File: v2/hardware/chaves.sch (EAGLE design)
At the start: 75 parts, among them IC1 40106N, IC2 7805DT

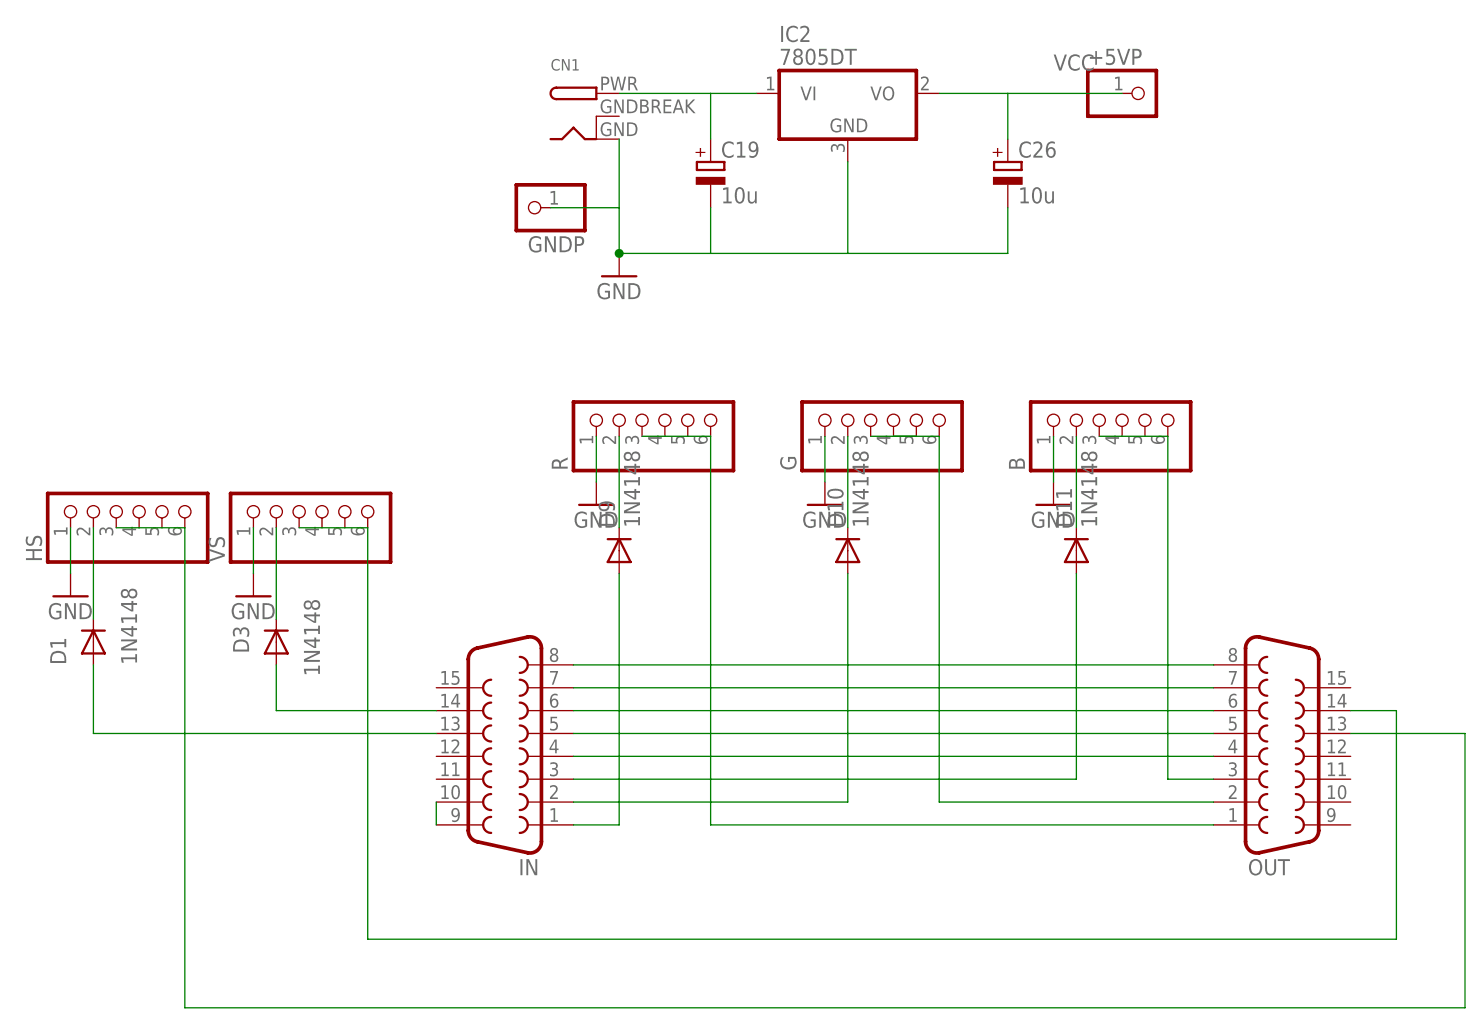
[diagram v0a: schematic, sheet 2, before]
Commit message: Revised gerbers for all versions
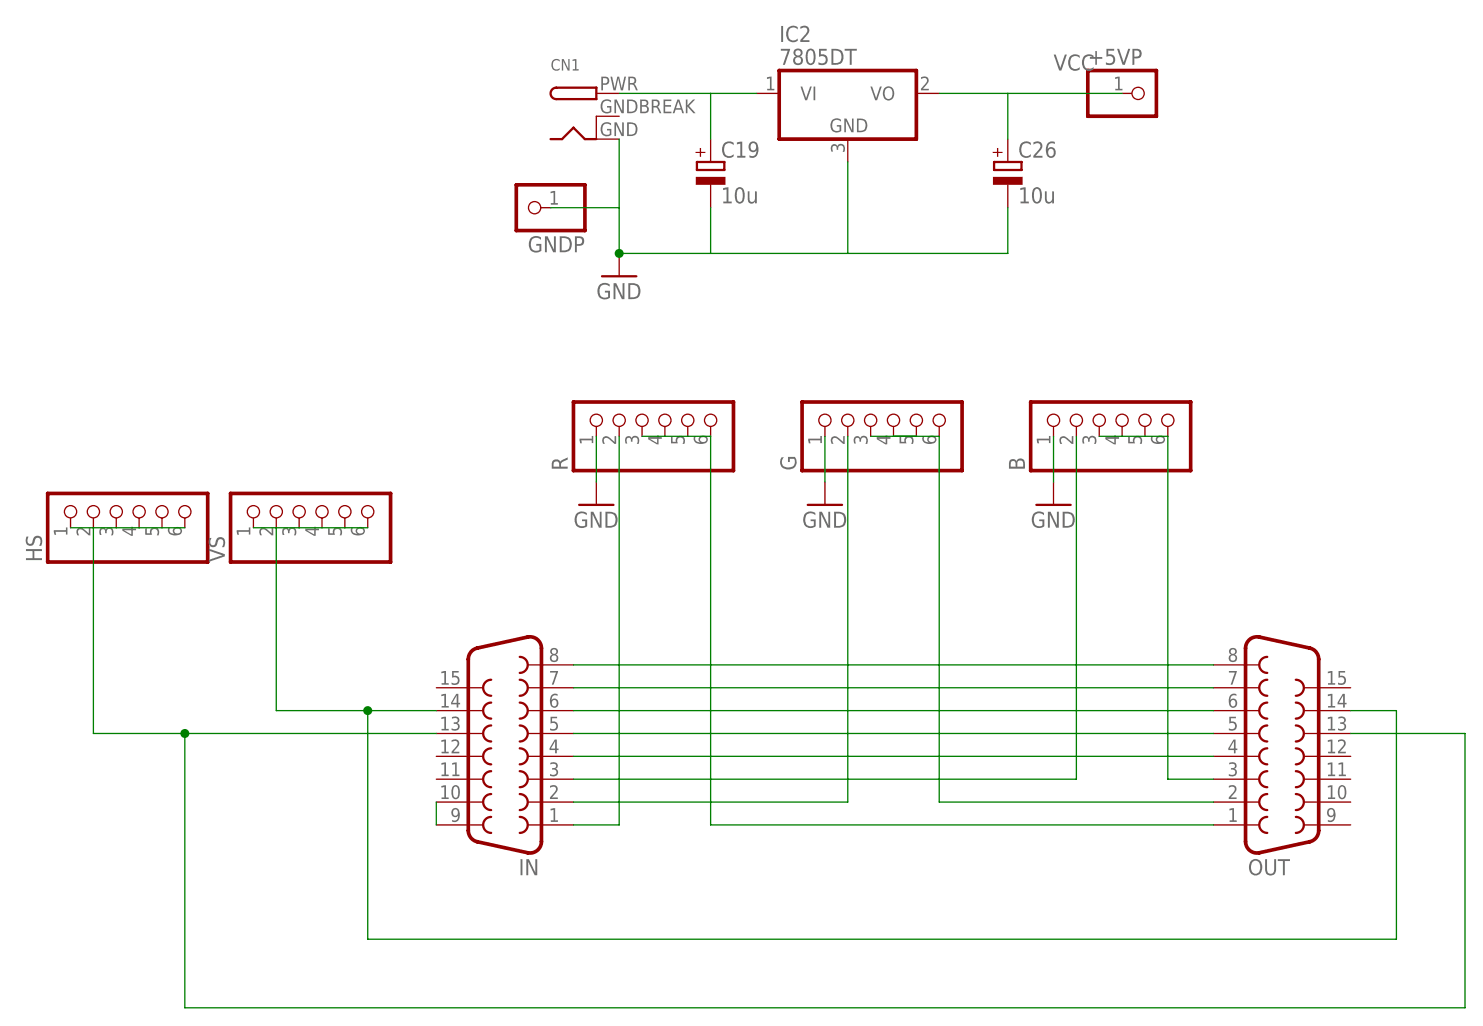
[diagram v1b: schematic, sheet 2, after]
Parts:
- removed D1, D10, D11, D3, D9: 1N4148, diode:1N4148DO35-7
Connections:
- removed net N$13: D9.C, R.2
- removed net N$20: D10.C, G.2
- removed net N$35: B.2, D11.C
- removed net N$60: D1.C, HS.2
- removed net N$62: D1.A, IN.13
- removed net N$63: D3.A, IN.14
- removed net N$64: D3.C, VS.2
- net GND: no longer HS.1, VS.1
- net N$12: now also R.2; no longer D9.A
- net N$15: now also G.2; no longer D10.A
- net N$25: now also B.2; no longer D11.A
- net N$54: now also IN.14, VS.1, VS.2
- net N$55: now also HS.1, HS.2, IN.13
